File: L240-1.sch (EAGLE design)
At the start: 15 parts, among them IC1 TINY13-20SSU, IC3 ACS712-LC, K1 G2R2, X4 MKDSN1,5/4-5,08

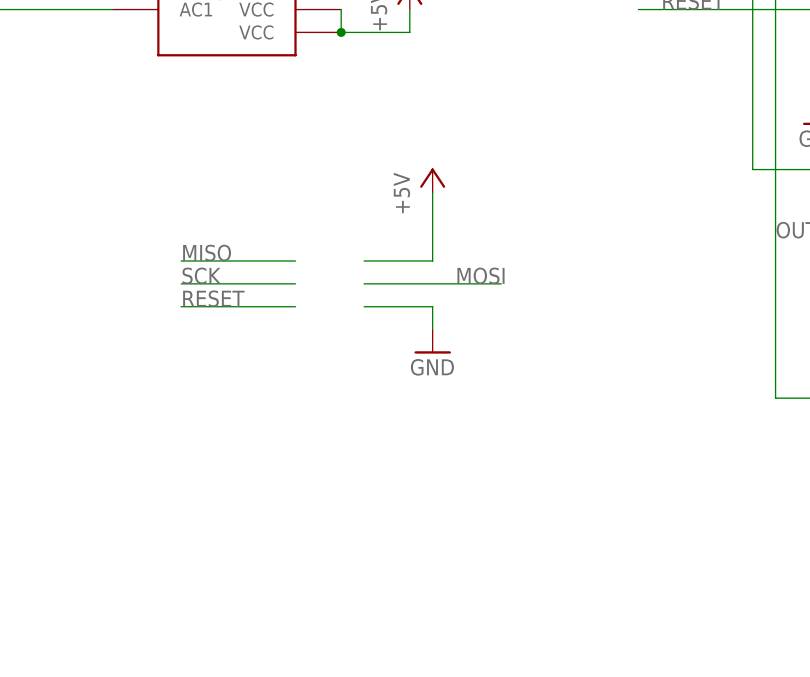
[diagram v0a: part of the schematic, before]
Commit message: v0.4
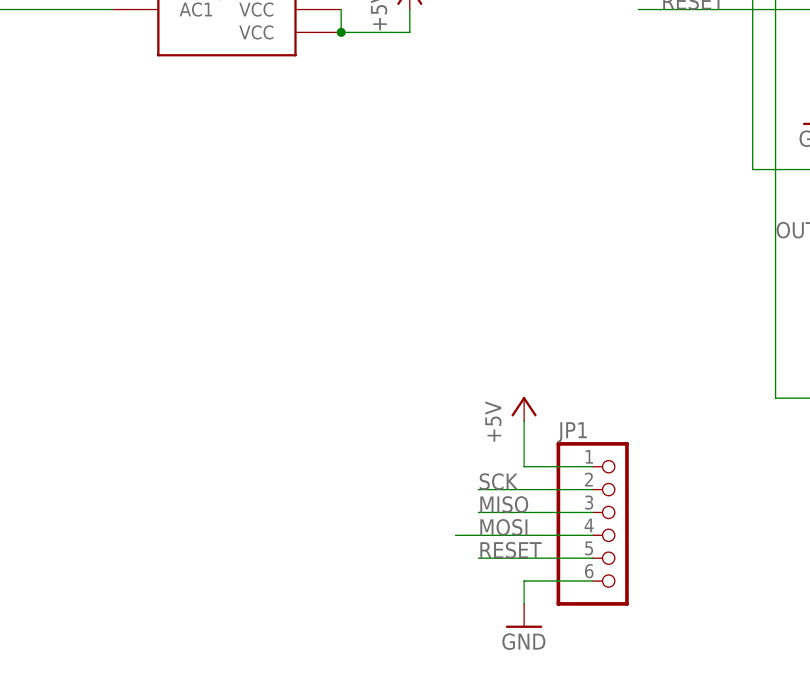
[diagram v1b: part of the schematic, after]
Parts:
- added JP1: (no value), pinhead:PINHD-1X6
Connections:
- net +5V: now also JP1.1
- net GND: now also JP1.6
- net MISO: now also JP1.3
- net MOSI: now also JP1.4
- net RESET: now also JP1.5
- net SCK: now also JP1.2
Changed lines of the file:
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@@
 <part name="GND2" library="supply1" deviceset="GND" device=""/>
 <part name="P+6" library="supply1" deviceset="+5V" device=""/>
+<part name="JP1" library="pinhead" library_urn="urn:adsk.eagle:library:325" deviceset="PINHD-1X6" device="" package3d_urn="urn:adsk.eagle:package:22472/2"/>
 </parts>
 <sheets>
@@
 <attribute name="VALUE" x="-1.016" y="99.441" size="1.778" layer="96"/>
 </instance>
-<instance part="GND22" gate="1" x="-7.62" y="25.4" smashed="yes">
-<attribute name="VALUE" x="-10.16" y="22.86" size="1.778" layer="96"/>
+<instance part="GND22" gate="1" x="2.54" y="-5.08" smashed="yes">
+<attribute name="VALUE" x="0" y="-7.62" size="1.778" layer="96"/>
 </instance>
 <instance part="GND3" gate="1" x="35.56" y="50.8" smashed="yes">
@@
 <attribute name="VALUE" x="33.02" y="83.82" size="1.778" layer="96" rot="R90"/>
 </instance>
-<instance part="P+5" gate="1" x="-7.62" y="45.72" smashed="yes">
-<attribute name="VALUE" x="-10.16" y="40.64" size="1.778" layer="96" rot="R90"/>
+<instance part="P+5" gate="1" x="2.54" y="20.32" smashed="yes">
+<attribute name="VALUE" x="0" y="15.24" size="1.778" layer="96" rot="R90"/>
 </instance>
 <instance part="C3" gate="G$1" x="7.62" y="104.14" smashed="yes">
@@
 <instance part="P+6" gate="1" x="-10.16" y="66.04" smashed="yes">
 <attribute name="VALUE" x="-12.7" y="60.96" size="1.778" layer="96" rot="R90"/>
+</instance>
+<instance part="JP1" gate="A" x="12.7" y="5.08" smashed="yes">
+<attribute name="NAME" x="6.35" y="15.875" size="1.778" layer="95"/>
+<attribute name="VALUE" x="6.35" y="-5.08" size="1.778" layer="96"/>
 </instance>
 </instances>
@@
 </segment>
 <segment>
-<pinref part="GND22" gate="1" pin="GND"/>
-<wire x1="-15.24" y1="30.48" x2="-7.62" y2="30.48" width="0.1524" layer="91"/>
-<wire x1="-7.62" y1="30.48" x2="-7.62" y2="27.94" width="0.1524" layer="91"/>
-</segment>
-<segment>
 <pinref part="IC1" gate="G$1" pin="GND"/>
 <wire x1="38.1" y1="60.96" x2="35.56" y2="60.96" width="0.1524" layer="91"/>
@@
 <pinref part="GND2" gate="1" pin="GND"/>
 <wire x1="-17.78" y1="81.28" x2="-12.7" y2="81.28" width="0.1524" layer="91"/>
+</segment>
+<segment>
+<pinref part="GND22" gate="1" pin="GND"/>
+<pinref part="JP1" gate="A" pin="6"/>
+<wire x1="2.54" y1="-2.54" x2="2.54" y2="0" width="0.1524" layer="91"/>
+<wire x1="2.54" y1="0" x2="10.16" y2="0" width="0.1524" layer="91"/>
 </segment>
 </net>
@@
 </segment>
 <segment>
-<wire x1="-15.24" y1="35.56" x2="-7.62" y2="35.56" width="0.1524" layer="91"/>
-<wire x1="-7.62" y1="35.56" x2="-7.62" y2="43.18" width="0.1524" layer="91"/>
-<pinref part="P+5" gate="1" pin="+5V"/>
-</segment>
-<segment>
 <pinref part="MD1" gate="G$1" pin="VCC@2"/>
 <pinref part="MD1" gate="G$1" pin="VCC@1"/>
@@
 <wire x1="-10.16" y1="60.96" x2="-10.16" y2="63.5" width="0.1524" layer="91"/>
 </segment>
+<segment>
+<pinref part="P+5" gate="1" pin="+5V"/>
+<pinref part="JP1" gate="A" pin="1"/>
+<wire x1="2.54" y1="17.78" x2="2.54" y2="12.7" width="0.1524" layer="91"/>
+<wire x1="2.54" y1="12.7" x2="10.16" y2="12.7" width="0.1524" layer="91"/>
+</segment>
 </net>
 <net name="MOSI" class="0">
 <segment>
-<wire x1="-15.24" y1="33.02" x2="0" y2="33.02" width="0.1524" layer="91"/>
-<label x="-5.08" y="33.02" size="1.778" layer="95"/>
+<wire x1="-5.08" y1="5.08" x2="10.16" y2="5.08" width="0.1524" layer="91"/>
+<label x="-2.54" y="5.08" size="1.778" layer="95"/>
+<pinref part="JP1" gate="A" pin="4"/>
 </segment>
 <segment>
@@
 <net name="MISO" class="0">
 <segment>
-<wire x1="-22.86" y1="35.56" x2="-35.56" y2="35.56" width="0.1524" layer="91"/>
-<label x="-35.56" y="35.56" size="1.778" layer="95"/>
+<wire x1="10.16" y1="7.62" x2="-2.54" y2="7.62" width="0.1524" layer="91"/>
+<label x="-2.54" y="7.62" size="1.778" layer="95"/>
+<pinref part="JP1" gate="A" pin="3"/>
 </segment>
 <segment>
@@
 <net name="SCK" class="0">
 <segment>
-<wire x1="-22.86" y1="33.02" x2="-35.56" y2="33.02" width="0.1524" layer="91"/>
-<label x="-35.56" y="33.02" size="1.778" layer="95"/>
+<wire x1="10.16" y1="10.16" x2="-2.54" y2="10.16" width="0.1524" layer="91"/>
+<label x="-2.54" y="10.16" size="1.778" layer="95"/>
+<pinref part="JP1" gate="A" pin="2"/>
 </segment>
 <segment>
@@
 <net name="RESET" class="0">
 <segment>
-<wire x1="-22.86" y1="30.48" x2="-35.56" y2="30.48" width="0.1524" layer="91"/>
-<label x="-35.56" y="30.48" size="1.778" layer="95"/>
-</segment>
-<segment>
+<wire x1="10.16" y1="2.54" x2="-2.54" y2="2.54" width="0.1524" layer="91"/>
+<label x="-2.54" y="2.54" size="1.778" layer="95"/>
+<pinref part="JP1" gate="A" pin="5"/>
+</segment>
+<segment>
